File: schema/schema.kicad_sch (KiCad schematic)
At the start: 15 parts, among them J1 MCU_ATmega328P_Module, J2 MCU_ATmega328P_Module, J3 LCD_1602_I2C, J4 MCU_ATmega328P_Module, J5 RF_433MHz_TX, J6 MCU_ATmega328P_Module, J7 RF_433MHz_RX, SW1 BTN_MORSE, SW2 BTN_SPEED_UP, SW3 BTN_SPEED_DOWN

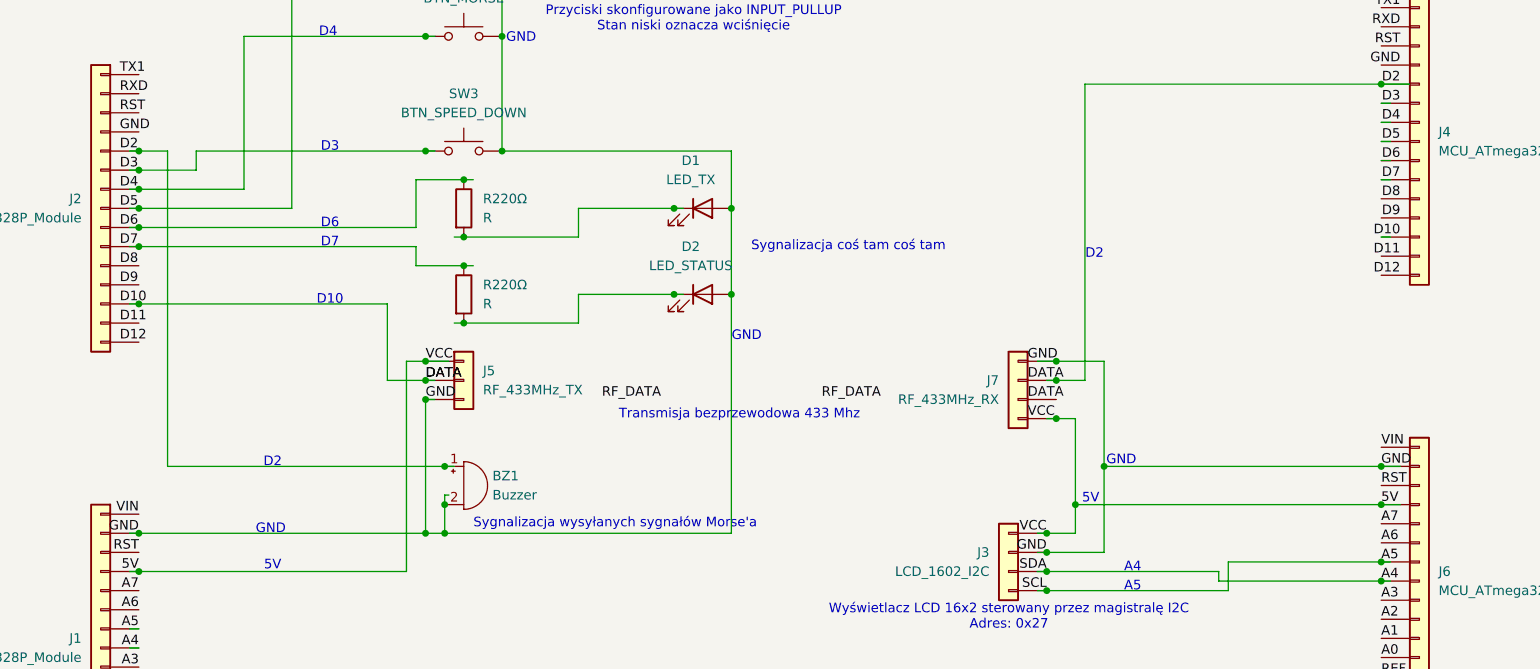
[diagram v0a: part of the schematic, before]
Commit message: Improve main schematics
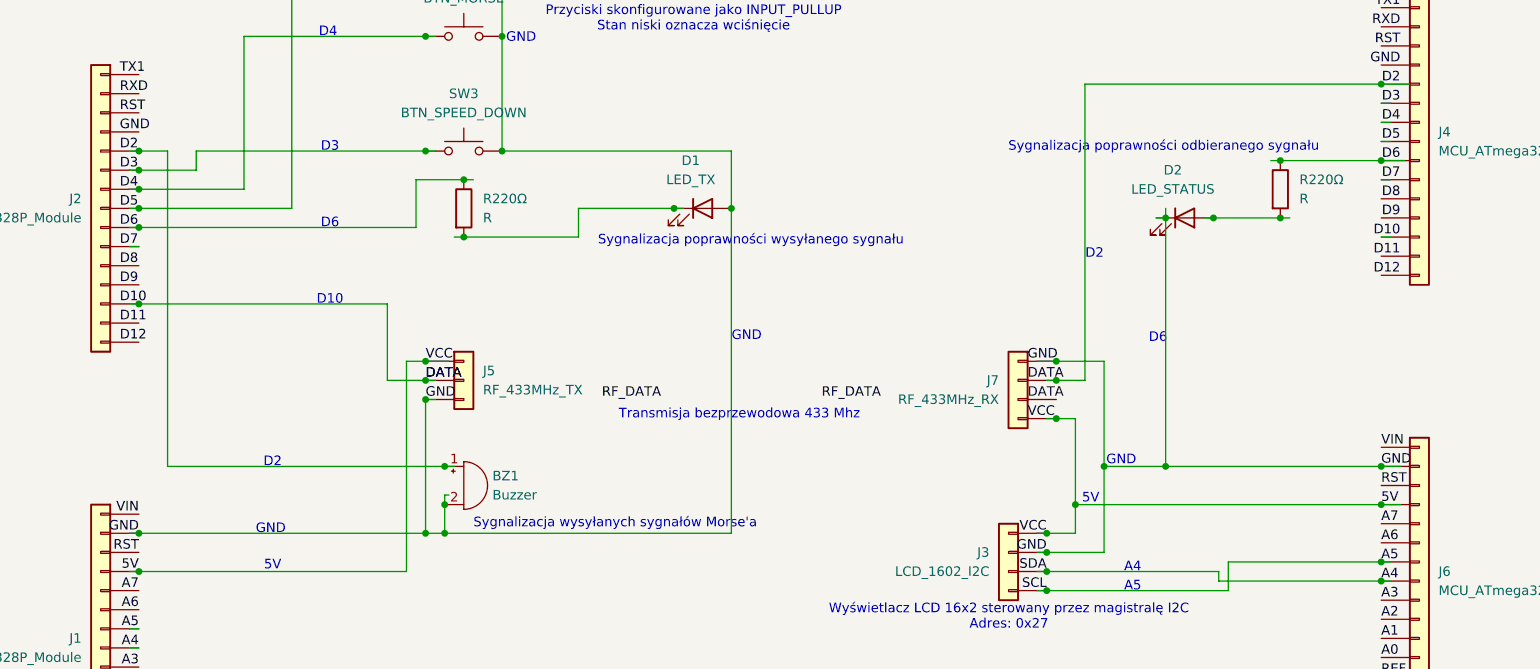
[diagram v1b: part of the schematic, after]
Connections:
- net D6: now also J4.9 (Pin_9), R220Ω.1
- net GND: now also D2.1 (K); no longer D2.2 (A)
- net at R220Ω.2: now also D2.2 (A); no longer D2.1 (K)
- net at J2.10 (Pin_10): no longer R220Ω.1
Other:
- note added: "Sygnalizacja poprawności odbieranego sygnału"
- note added: "Sygnalizacja poprawności wysyłanego sygnału"
- note removed: "D7"
- note removed: "Sygnalizacja coś tam coś tam"
- moved on the sheet: D2, R220Ω
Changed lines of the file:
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@@
+		)
+	)
+	(text "Sygnalizacja poprawności odbieranego sygnału"
+		(exclude_from_sim no)
+		(at 197.866 55.372 0)
+		(effects
+			(font
+				(size 1.27 1.27)
+			)
 		)
 	)
@@
 		)
 	)
-	(text "D7"
+	(text "D6"
 		(exclude_from_sim no)
-		(at 87.0656 68.072 0)
+		(at 197.104 80.772 0)
 		(effects
 			(font
@@
 		)
 	)
-	(text "Sygnalizacja coś tam coś tam"
+	(text "Sygnalizacja poprawności wysyłanego sygnału"
 		(exclude_from_sim no)
-		(at 155.956 68.58 0)
+		(at 143.002 67.818 0)
 		(effects
 			(font
@@
 	)
 	(junction
-		(at 140.4056 74.93)
+		(at 198.12 64.77)
+		(diameter 0)
+		(color 0 0 0 0)
+	)
+	(junction
+		(at 213.36 57.15)
 		(diameter 0)
 		(color 0 0 0 0)
@@
 	)
 	(junction
-		(at 132.7856 74.93)
-		(diameter 0)
-		(color 0 0 0 0)
-	)
-	(junction
 		(at 102.3056 106.68)
 		(diameter 0)
@@
 	)
 	(junction
+		(at 226.7656 57.15)
+		(diameter 0)
+		(color 0 0 0 0)
+	)
+	(junction
 		(at 182.3156 114.3)
 		(diameter 0)
@@
 	)
 	(junction
+		(at 198.12 97.79)
+		(diameter 0)
+		(color 0 0 0 1)
+	)
+	(junction
 		(at 104.8456 67.31)
 		(diameter 0)
@@
 	)
 	(junction
+		(at 204.47 64.77)
+		(diameter 0)
+		(color 0 0 0 0)
+	)
+	(junction
 		(at 61.6656 111.76)
 		(diameter 0)
@@
 	)
 	(junction
-		(at 104.8456 78.74)
+		(at 213.36 64.77)
 		(diameter 0)
 		(color 0 0 0 0)
@@
 	)
 	(junction
-		(at 61.6656 68.58)
-		(diameter 0)
-		(color 0 0 0 0)
-	)
-	(junction
 		(at 99.7656 25.4)
 		(diameter 0)
@@
 	)
 	(junction
-		(at 104.8456 71.12)
-		(diameter 0)
-		(color 0 0 0 0)
-	)
-	(junction
 		(at 99.7656 106.68)
 		(diameter 0)
@@
 	(wire
 		(pts
+			(xy 212.09 57.15) (xy 213.36 57.15)
+		)
+		(stroke
+			(width 0)
+			(type default)
+		)
+	)
+	(wire
+		(pts
 			(xy 61.6656 60.96) (xy 75.6356 60.96)
 		)
@@
 	(wire
 		(pts
-			(xy 228.0356 57.15) (xy 226.7656 57.15)
-		)
-		(stroke
-			(width 0)
-			(type default)
-		)
-	)
-	(wire
-		(pts
 			(xy 61.6656 58.42) (xy 69.2856 58.42)
 		)
@@
 	(wire
 		(pts
-			(xy 189.9356 97.79) (xy 226.7656 97.79)
+			(xy 189.9356 97.79) (xy 198.12 97.79)
 		)
 		(stroke
@@
 	(wire
 		(pts
-			(xy 104.8456 71.12) (xy 106.1156 71.12)
-		)
-		(stroke
-			(width 0)
-			(type default)
-		)
-	)
-	(wire
-		(pts
 			(xy 65.4756 55.88) (xy 65.4756 97.79)
 		)
@@
 	(wire
 		(pts
+			(xy 198.12 64.77) (xy 198.12 97.79)
+		)
+		(stroke
+			(width 0)
+			(type default)
+		)
+	)
+	(wire
+		(pts
 			(xy 181.0456 111.76) (xy 182.3156 111.76)
 		)
@@
 	(wire
 		(pts
-			(xy 104.8456 78.74) (xy 120.0856 78.74)
-		)
-		(stroke
-			(width 0)
-			(type default)
-		)
-	)
-	(wire
-		(pts
 			(xy 226.7656 46.99) (xy 230.5756 46.99)
 		)
@@
 	(wire
 		(pts
-			(xy 103.5756 78.74) (xy 104.8456 78.74)
-		)
-		(stroke
-			(width 0)
-			(type default)
-		)
-	)
-	(wire
-		(pts
 			(xy 61.6656 76.2) (xy 94.6856 76.2)
 		)
@@
 	(wire
 		(pts
+			(xy 203.2 64.77) (xy 204.47 64.77)
+		)
+		(stroke
+			(width 0)
+			(type default)
+		)
+	)
+	(wire
+		(pts
 			(xy 186.1256 102.87) (xy 226.7656 102.87)
 		)
@@
 	(wire
 		(pts
+			(xy 213.36 64.77) (xy 214.63 64.77)
+		)
+		(stroke
+			(width 0)
+			(type default)
+		)
+	)
+	(wire
+		(pts
 			(xy 189.9356 97.79) (xy 189.9356 109.22)
 		)
@@
 	(wire
 		(pts
-			(xy 61.6656 68.58) (xy 98.4956 68.58)
-		)
-		(stroke
-			(width 0)
-			(type default)
-		)
-	)
-	(wire
-		(pts
 			(xy 60.3956 55.88) (xy 61.6656 55.88)
 		)
@@
 	(wire
 		(pts
+			(xy 198.12 97.79) (xy 226.7656 97.79)
+		)
+		(stroke
+			(width 0)
+			(type default)
+			(color 72 72 72 1)
+		)
+	)
+	(wire
+		(pts
+			(xy 204.47 64.77) (xy 213.36 64.77)
+		)
+		(stroke
+			(width 0)
+			(type default)
+		)
+	)
+	(wire
+		(pts
 			(xy 205.1756 113.03) (xy 226.7656 113.03)
 		)
@@
 	(wire
 		(pts
-			(xy 120.0856 74.93) (xy 132.7856 74.93)
-		)
-		(stroke
-			(width 0)
-			(type default)
-		)
-	)
-	(wire
-		(pts
 			(xy 226.7656 113.03) (xy 228.0356 113.03)
 		)
@@
 	(wire
 		(pts
+			(xy 213.36 57.15) (xy 226.7656 57.15)
+		)
+		(stroke
+			(width 0)
+			(type default)
+		)
+	)
+	(wire
+		(pts
 			(xy 181.0456 83.82) (xy 183.5856 83.82)
 		)
@@
 	(wire
 		(pts
-			(xy 140.4056 106.68) (xy 140.4056 74.93)
+			(xy 140.4056 63.5) (xy 140.4056 106.68)
 		)
 		(stroke
@@
 	(wire
 		(pts
-			(xy 132.7856 74.93) (xy 134.0556 74.93)
+			(xy 196.85 64.77) (xy 198.12 64.77)
 		)
 		(stroke
@@
 	(wire
 		(pts
-			(xy 98.4956 71.12) (xy 104.8456 71.12)
-		)
-		(stroke
-			(width 0)
-			(type default)
-		)
-	)
-	(wire
-		(pts
 			(xy 69.2856 55.88) (xy 99.7656 55.88)
 		)
@@
 	(wire
 		(pts
-			(xy 120.0856 78.74) (xy 120.0856 74.93)
-		)
-		(stroke
-			(width 0)
-			(type default)
-		)
-	)
-	(wire
-		(pts
 			(xy 181.0456 106.68) (xy 182.3156 106.68)
 		)
@@
 	(wire
 		(pts
-			(xy 140.4056 63.5) (xy 140.4056 74.93)
+			(xy 198.12 63.5) (xy 198.12 64.77)
+		)
+		(stroke
+			(width 0)
+			(type default)
+		)
+	)
+	(wire
+		(pts
+			(xy 182.3156 109.22) (xy 189.9356 109.22)
 		)
 		(stroke
@@
 	(wire
 		(pts
-			(xy 182.3156 109.22) (xy 189.9356 109.22)
-		)
-		(stroke
-			(width 0)
-			(type default)
-			(color 72 72 72 1)
+			(xy 226.7656 57.15) (xy 229.87 57.15)
+		)
+		(stroke
+			(width 0)
+			(type default)
 		)
 	)
@@
 		(pts
 			(xy 98.4956 59.69) (xy 104.8456 59.69)
-		)
-		(stroke
-			(width 0)
-			(type default)
-		)
-	)
-	(wire
-		(pts
-			(xy 98.4956 68.58) (xy 98.4956 71.12)
 		)
 		(stroke
@@
 	(symbol
 		(lib_id "Device:LED")
-		(at 136.5956 74.93 0)
+		(at 200.66 64.77 0)
 		(unit 1)
 		(body_style 1)
@@
 		(fields_autoplaced yes)
 		(property "Reference" "D2"
-			(at 135.0081 68.58 0)
+			(at 199.0725 58.42 0)
 			(show_name no)
 			(do_not_autoplace no)
@@
 		)
 		(property "Value" "LED_STATUS"
-			(at 135.0081 71.12 0)
+			(at 199.0725 60.96 0)
 			(show_name no)
 			(do_not_autoplace no)
@@
 		)
 		(property "Footprint" ""
-			(at 136.5956 74.93 0)
+			(at 200.66 64.77 0)
 			(hide yes)
 			(show_name no)
@@
 		)
 		(property "Datasheet" ""
-			(at 136.5956 74.93 0)
+			(at 200.66 64.77 0)
 			(hide yes)
 			(show_name no)
@@
 		)
 		(property "Description" "Light emitting diode"
-			(at 136.5956 74.93 0)
+			(at 200.66 64.77 0)
 			(hide yes)
 			(show_name no)
@@
 		)
 		(property "Sim.Pins" "1=K 2=A"
-			(at 136.5956 74.93 0)
+			(at 200.66 64.77 0)
 			(hide yes)
 			(show_name no)
@@
 	(symbol
 		(lib_id "Device:R")
-		(at 104.8456 74.93 0)
+		(at 213.36 60.96 0)
 		(unit 1)
 		(body_style 1)
@@
 		(fields_autoplaced yes)
 		(property "Reference" "R220Ω"
-			(at 107.3856 73.6599 0)
+			(at 215.9 59.6899 0)
 			(show_name no)
 			(do_not_autoplace no)
@@
 		)
 		(property "Value" "R"
-			(at 107.3856 76.1999 0)
+			(at 215.9 62.2299 0)
 			(show_name no)
 			(do_not_autoplace no)
@@
 		)
 		(property "Footprint" ""
-			(at 103.0676 74.93 90)
+			(at 211.582 60.96 90)
 			(hide yes)
 			(show_name no)
@@
 		)
 		(property "Datasheet" ""
-			(at 104.8456 74.93 0)
+			(at 213.36 60.96 0)
 			(hide yes)
 			(show_name no)
@@
 		)
 		(property "Description" "Resistor"
-			(at 104.8456 74.93 0)
-			(hide yes)
-			(show_name no)
+			(at 213.36 60.96 0)
+			(hide yes)
+			(show_name no)
